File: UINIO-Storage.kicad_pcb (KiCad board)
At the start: 2 copper layers, 60 x 39.5 mm, 46 parts, among them J1 Conn_01x04_Pin, J2 Conn_01x04_Pin, J3 Conn_01x06_Pin, J4 Conn_01x06_Pin, J5 Conn_01x06_Pin, U1 I2C-24-EEPROM-SOIC8, U2 I2C-24-EEPROM-TSSOP8, U3 SPI-25-Flash-SOIC8, U4 ME6211, U5 SPI-25-Flash-WSON8

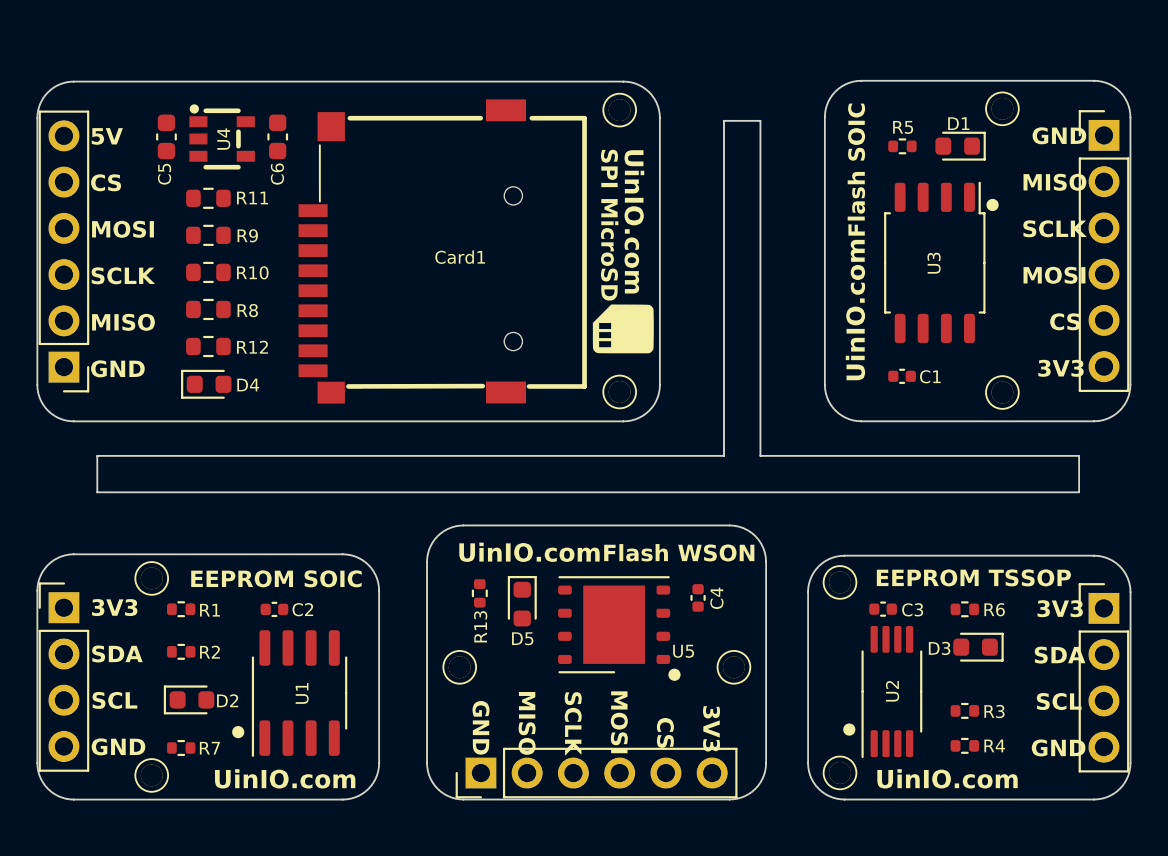
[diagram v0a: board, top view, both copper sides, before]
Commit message: Finish PCB Layout.
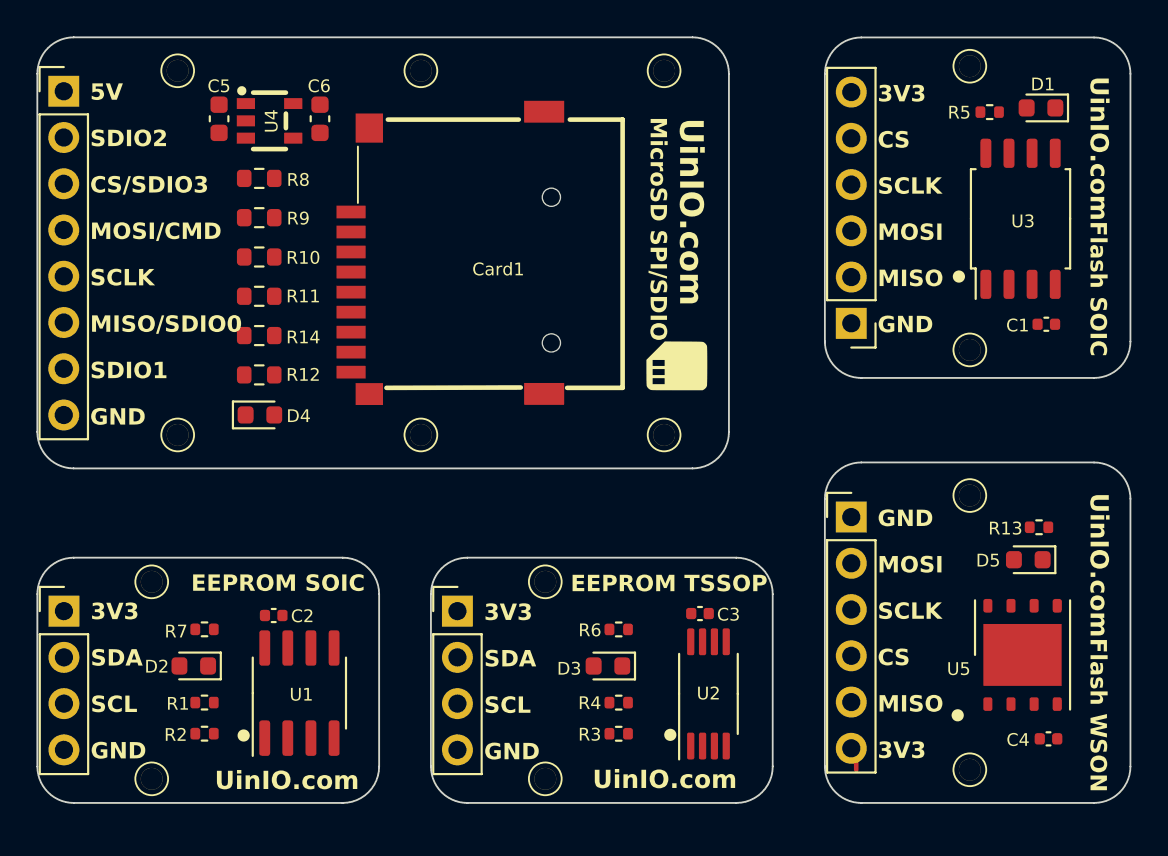
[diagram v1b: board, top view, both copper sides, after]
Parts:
- removed the HOLE** at (165.7, 113.1)
- removed the HOLE** at (165.7, 123.6)
- added HOLE**: Hole-1mm, Uinio:Hole-1mm, F.Cu at (142.6, 105.0)
- added HOLE**: Hole-1mm, Uinio:Hole-1mm, F.Cu at (129.3, 105.0)
- added HOLE**: Hole-1mm, Uinio:Hole-1mm, F.Cu at (142.6, 85.0)
- added HOLE**: Hole-1mm, Uinio:Hole-1mm, F.Cu at (129.3, 85.0)
- added HOLE**: Hole-1mm, Uinio:Hole-1mm, F.Cu at (149.5, 123.9)
- added HOLE**: Hole-1mm, Uinio:Hole-1mm, F.Cu at (149.5, 113.1)
- added R14: 10K, Resistor_SMD:R_0603_1608Metric, F.Cu at (133.8, 99.5)
- J4: value Conn_01x06_Pin -> Conn_01x08_Pin; footprint Connector_PinHeader_2.54mm:PinHeader_1x06_P2.54mm_Vertical -> Connector_PinHeader_2.54mm:PinHeader_1x08_P2.54mm_Vertical
- moved J2 35.5 mm to (144.7, 114.7)
- moved R13 30.9 mm to (176.6, 110.1), turned to 0 degrees
- moved HOLE** 29.6 mm to (172.8, 108.3), turned to -90 degrees
- moved D5 27.9 mm to (176.0, 111.9), turned to 180 degrees
- moved J5 24.7 mm to (166.3, 109.5), turned to 0 degrees
- moved U5 22.5 mm to (175.7, 117.1), turned to 90 degrees
- moved C4 20.7 mm to (177.1, 121.7), turned to 0 degrees
- moved D3 20.2 mm to (152.9, 117.7)
- moved R4 19.2 mm to (153.5, 119.7), turned to 0 degrees
- moved R3 19.0 mm to (153.5, 121.4), turned to 180 degrees
- moved R6 19.0 mm to (153.5, 115.7), turned to 180 degrees
- moved HOLE** 18.0 mm to (172.8, 84.8), turned to 180 degrees
- moved J3 17.3 mm to (166.3, 98.9), turned to 180 degrees
- moved J4 15.1 mm to (123.0, 86.1), turned to 0 degrees
- moved HOLE** 14.1 mm to (172.8, 123.4), turned to -90 degrees
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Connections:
- C5 pad 1: /SD-GND -> /SPI/SDIO-GND
- C5 pad 2: /SD-5V -> /SPI/SDIO-5V
- C6 pad 1: /SD-GND -> /SPI/SDIO-GND
- C6 pad 2: /SD-3.3V -> /SPI/SDIO-3.3V
- Card1 pad 1: unconnected-(Card1-DAT2-Pad1) -> /SDIO-2
- Card1 pad 2: /SD-CS -> /SPI-CS/SDIO-3
- Card1 pad 3: /SD-MOSI -> /SPI-MOSI/SDIO-CMD
- Card1 pad 4: /SD-3.3V -> /SPI/SDIO-3.3V
- Card1 pad 5: /SD-SCLK -> /SPI/SDIO-SCLK
- Card1 pad 6: /SD-GND -> /SPI/SDIO-GND
- Card1 pad 7: /SD-MISO -> /SPI-MISO/SDIO-0
- Card1 pad 8: unconnected-(Card1-DAT1-Pad8) -> /SDIO1
- D4 pad 1: /SD-GND -> /SPI/SDIO-GND
- J1 pad 2: /EEPROM-SOIC8-SDA -> /EEPROM-SOIC8-SCL
- J1 pad 3: /EEPROM-SOIC8-SCL -> /EEPROM-SOIC8-SDA
- J2 pad 2: /EEPROM-TSSOP8-SDA -> /EEPROM-TSSOP8-SCL
- J2 pad 3: /EEPROM-TSSOP8-SCL -> /EEPROM-TSSOP8-SDA
- J3 pad 2: /Flash-SOIC8-MISO -> /Flash-SOIC8-CS
- J3 pad 3: /Flash-SOIC8-MOSI -> /Flash-SOIC8-MISO
- J3 pad 4: /Flash-SOIC8-CLK -> /Flash-SOIC8-MOSI
- J3 pad 5: /Flash-SOIC8-CS -> /Flash-SOIC8-CLK
- J4 pad 1: /SD-GND -> /SPI/SDIO-5V
- J4 pad 2: /SD-MISO -> /SDIO-2
- J4 pad 3: /SD-SCLK -> /SPI-CS/SDIO-3
- J4 pad 4: /SD-MOSI -> /SPI-MOSI/SDIO-CMD
- J4 pad 5: /SD-CS -> /SPI/SDIO-SCLK
- J4 pad 6: /SD-5V -> /SPI-MISO/SDIO-0
- J5 pad 2: /Flash-WSON8-MISO -> /Flash-WSON8-MOSI
- J5 pad 3: /Flash-WSON8-MOSI -> /Flash-WSON8-CLK
- J5 pad 4: /Flash-WSON8-CLK -> /Flash-WSON8-CS
- J5 pad 5: /Flash-WSON8-CS -> /Flash-WSON8-MISO
- R10 pad 2: /SD-SCLK -> /SPI-MOSI/SDIO-CMD
- R11 pad 2: /SD-CS -> /SPI-MISO/SDIO-0
- R12 pad 1: /SD-3.3V -> /SPI/SDIO-3.3V
- R8 pad 2: /SD-MISO -> /SDIO-2
- R9 pad 2: /SD-MOSI -> /SPI-CS/SDIO-3
- U4 pad 1: /SD-5V -> /SPI/SDIO-5V
- U4 pad 2: /SD-GND -> /SPI/SDIO-GND
- U4 pad 3: /SD-5V -> /SPI/SDIO-5V
- U4 pad 5: /SD-3.3V -> /SPI/SDIO-3.3V
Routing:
- net /Flash-WSON8-3.3V: track 0.00 -> 1.69 mm
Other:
- board size 60 x 39.5 mm -> 60 x 42 mm
- board text added: "CS/SDIO3"
- board text added: "MISO/SDIO0"
- board text added: "MOSI/CMD"
- board text added: "MicroSD SPI/SDIO"
- board text added: "SDIO1"
- board text added: "SDIO2"
- board text removed: "SPI MicroSD"

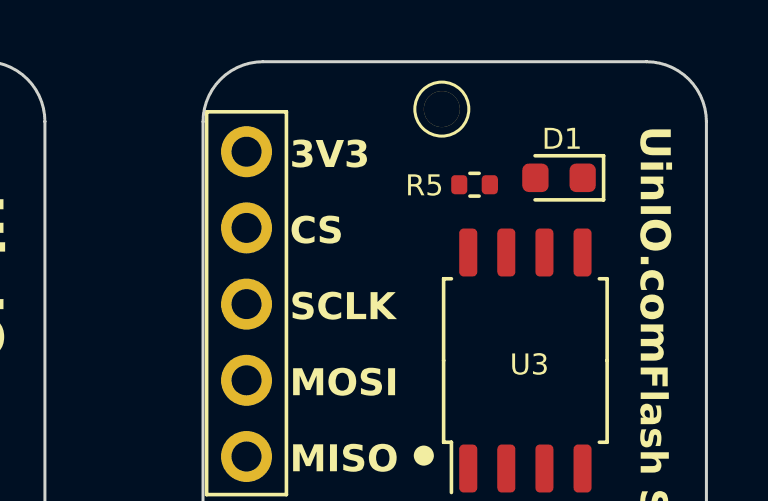
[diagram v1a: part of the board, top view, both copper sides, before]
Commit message: Finish PCB Layout.
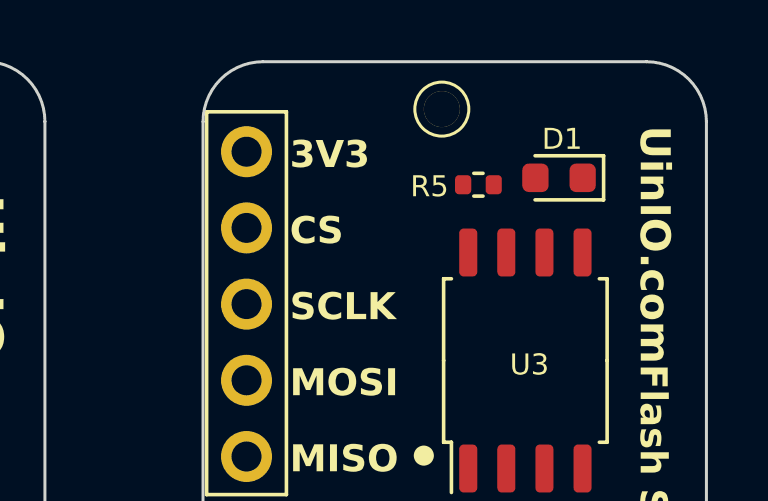
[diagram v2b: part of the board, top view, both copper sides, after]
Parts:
- moved R5 0.13 mm to (174.0, 87.3)
